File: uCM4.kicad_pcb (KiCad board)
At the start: 2 copper layers, 55 x 48 mm, 81 parts, among them IC1 MAX17048G+, J10 USB_C_Receptacle, J2 Micro_SD_Card_Det, J4 Conn_01x04, J5 DummyJ, J6 DummyJ, Q2 SI2369DS, U1 BNO055, U18 RT9742GGJ5, U2 SN74LVC1G07DBVR, U3 TPS3839DBZ, U4 TPS61022, U5 TPD2EUSB30, U6 TP4057, U7 HC-PM254-5.0H-2X7PS, U8 ADAU7002ACBZ-R7, U9 HC-PM254-5.0H-2X7PS

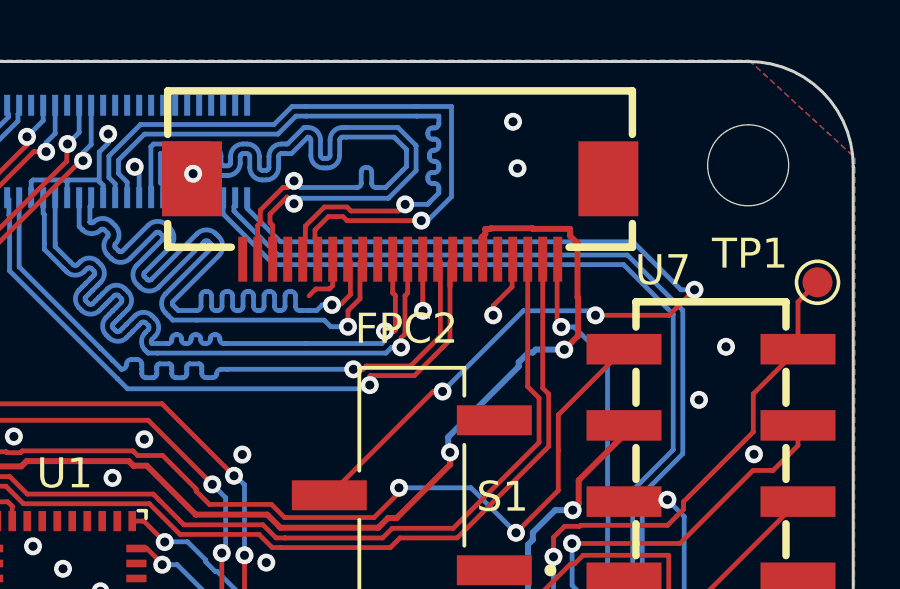
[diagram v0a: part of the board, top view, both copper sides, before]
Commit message: Production ready files.
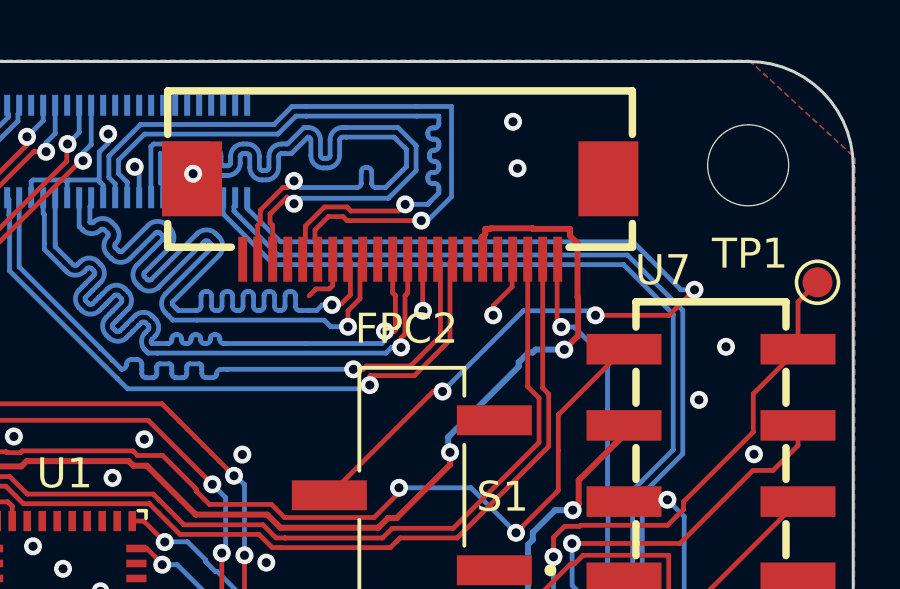
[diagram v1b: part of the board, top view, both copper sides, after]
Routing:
- net /CAM1_D3_P: track 23.2 -> 22.4 mm
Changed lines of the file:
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@@
 			)
 		)
-		(property "LCSC Part" "C42163135"
+		(property "LCSC Part #" "C42163135"
 			(at 0 0 90)
 			(unlocked yes)
@@
 		(sheetname "/")
 		(sheetfile "uCM4.kicad_sch")
-		(attr exclude_from_pos_files)
+		(attr exclude_from_pos_files exclude_from_bom)
 		(fp_circle
 			(center 0 0)
@@
 		(sheetname "/")
 		(sheetfile "uCM4.kicad_sch")
-		(attr exclude_from_pos_files)
+		(attr exclude_from_pos_files exclude_from_bom)
 		(fp_circle
 			(center 0 0)
@@
 			)
 		)
-		(property "LCSC Part" "C42163135"
+		(property "LCSC Part #" "C42163135"
 			(at 0 0 270)
 			(unlocked yes)
@@
 		(sheetname "/")
 		(sheetfile "uCM4.kicad_sch")
-		(attr exclude_from_pos_files)
+		(attr exclude_from_pos_files exclude_from_bom)
 		(fp_circle
 			(center 0 0)
@@
 		(sheetname "/")
 		(sheetfile "uCM4.kicad_sch")
-		(attr exclude_from_pos_files)
+		(attr exclude_from_pos_files exclude_from_bom)
 		(fp_circle
 			(center 0 0)
@@
 		(sheetname "/")
 		(sheetfile "uCM4.kicad_sch")
-		(attr exclude_from_pos_files)
+		(attr exclude_from_pos_files exclude_from_bom)
 		(fp_circle
 			(center 0 0)
@@
 			)
 		)
-		(property "LCSC#" "C424649"
+		(property "LCSC#" "C597931"
+			(at 0 0 180)
+			(unlocked yes)
+			(layer "B.Fab")
+			(hide yes)
+			(effects
+				(font
+					(size 1 1)
+					(thickness 0.15)
+				)
+				(justify mirror)
+			)
+		)
+		(property "LCSC Part #" "C597931"
 			(at 0 0 180)
 			(unlocked yes)
@@
 			)
 		)
-		(property "LCSC#" "C424649"
+		(property "LCSC#" "C597931"
+			(at 0 0 180)
+			(unlocked yes)
+			(layer "B.Fab")
+			(hide yes)
+			(effects
+				(font
+					(size 1 1)
+					(thickness 0.15)
+				)
+				(justify mirror)
+			)
+		)
+		(property "LCSC Part #" "C597931"
 			(at 0 0 180)
 			(unlocked yes)
@@
 		(sheetname "/")
 		(sheetfile "uCM4.kicad_sch")
-		(attr smd exclude_from_pos_files)
+		(attr smd exclude_from_pos_files exclude_from_bom)
 		(fp_line
 			(start 0 -3.5)
@@
 		(width 0.16)
 		(layer "F.Cu")
-		(net 33)
-	)
-	(segment
-		(start 162.5 92.55)
-		(end 162.5 91.72)
-		(width 0.16)
-		(layer "F.Cu")
